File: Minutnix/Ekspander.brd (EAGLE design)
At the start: 215.2 x 44.1 mm, 14 parts, among them X1 FH12-12S-0.5S_THINNER, X6 JST-XH-03-PIN-LONG-PAD

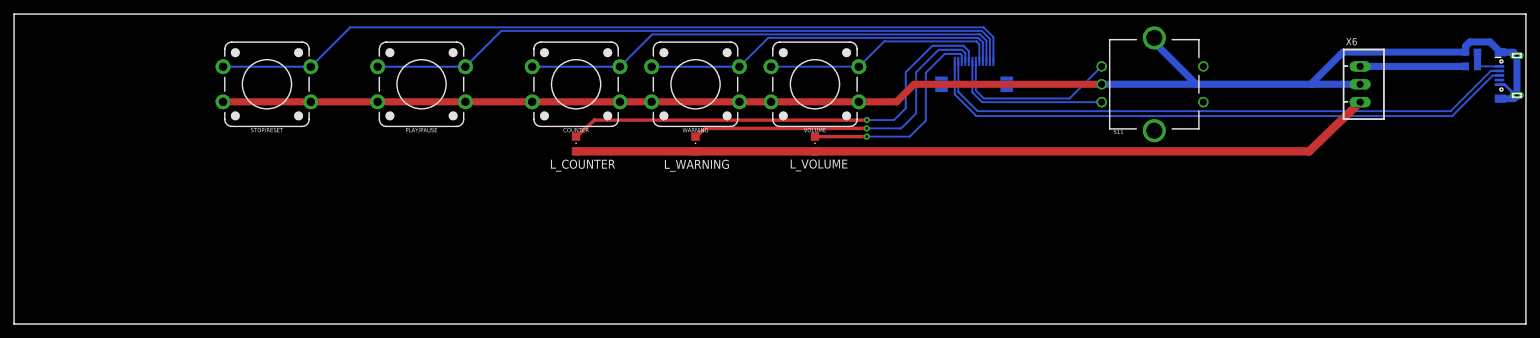
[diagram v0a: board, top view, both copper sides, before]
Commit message: Probably final routing of Expander board
DRC 8mils clean
libs actualisation
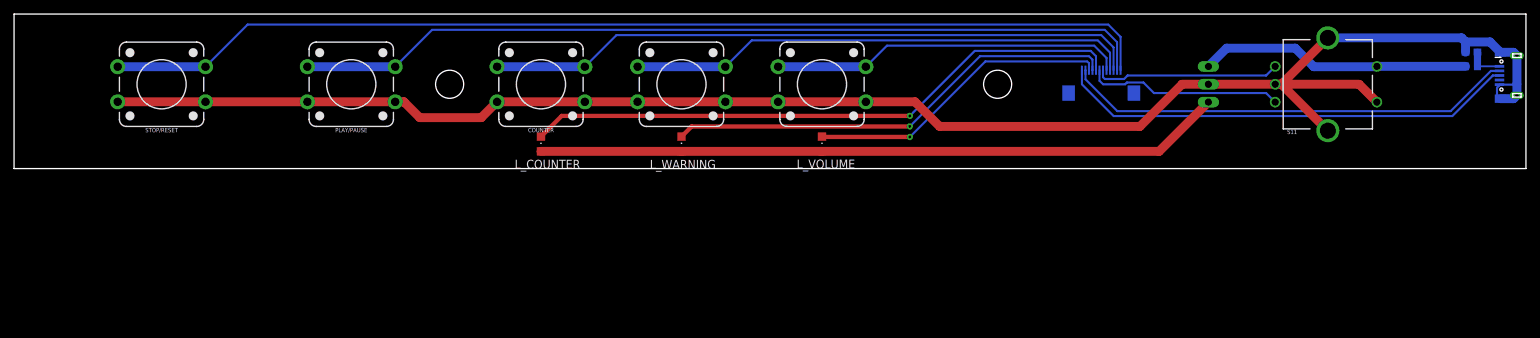
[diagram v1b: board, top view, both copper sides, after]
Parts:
- PLAY/PAUSE: device SparkFun-Switches:TACTILE_SWITCH_PTH_12MM -> MySparkFun-Switches:TACTILE_SWITCH_PTH_12MM
- moved S11 24.7 mm to (187.0, -10.0)
- moved X6 21.6 mm to (170.0, -10.0), flipped to the bottom
- moved X1 18.1 mm to (154.8, -11.2)
- moved STOP/RESET 15.0 mm to (21.0, -10.0)
- moved PLAY/PAUSE 10.0 mm to (48.0, -10.0)
- moved COUNTER 5.00 mm to (75.0, -10.0)
- moved L_COUNTER 5.00 mm to (75.0, -18.5)
- moved L_WARNING 2.00 mm to (95.0, -18.5)
- moved WARNING 2.00 mm to (95.0, -10.0)
- moved L_VOLUME 1.00 mm to (115.0, -18.5)
- moved VOLUME 1.00 mm to (115.0, -10.0)
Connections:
- net +5V: now also S11.SW-
- net GND: now also COUNTER.4, PLAY/PAUSE.4, S11.P$3, S11.P$4, S11.SW+, STOP/RESET.4, VOLUME.4, WARNING.4
- net N$2: now also STOP/RESET.2
- net N$3: now also PLAY/PAUSE.2
- net N$4: now also COUNTER.2
- net N$5: now also WARNING.2
- net N$6: now also VOLUME.2
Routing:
- net N$2: track 116.0 -> 150.7 mm
- net VCC: track 131.4 -> 97.9 mm
- net N$3: track 92.9 -> 122.1 mm
- net GND: track 272.6 -> 248.1 mm
- net +5V: track 15.0 -> 38.8 mm
- net N$4: track 69.9 -> 93.6 mm
- net N$10: track 66.0 -> 86.4 mm
- net N$7: track 84.9 -> 64.5 mm
- net N$5: track 51.8 -> 72.0 mm
- net N$9: track 85.9 -> 65.7 mm
- net N$6: track 33.8 -> 50.5 mm
- net N$11: track 48.2 -> 64.9 mm
- net N$12: track 30.7 -> 43.6 mm
- net N$8: track 23.4 -> 28.0 mm
- net N$1: track 24.4 -> 26.4 mm
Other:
- board size 215.2 x 44.1 mm -> 215.2 x 22 mm
